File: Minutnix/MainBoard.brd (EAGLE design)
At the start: 222.3 x 73.3 mm, 121 parts, among them IC3 TP4056, IC7 FT232RL, Q4 32.768kHz, X1 FH12-12S-0.5S_THINNER, X2 JST-XH-03-PIN-LONG-PAD, X4 JST-XH-03-PIN-LONG-PAD

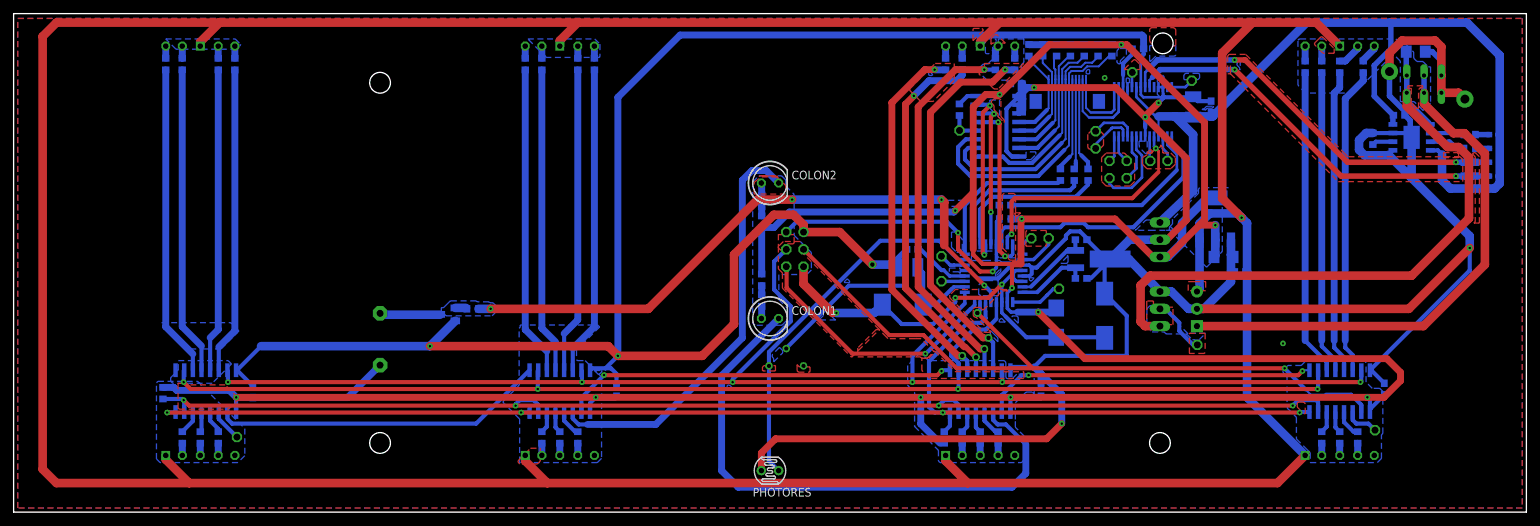
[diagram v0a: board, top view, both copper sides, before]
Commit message: Many final changes
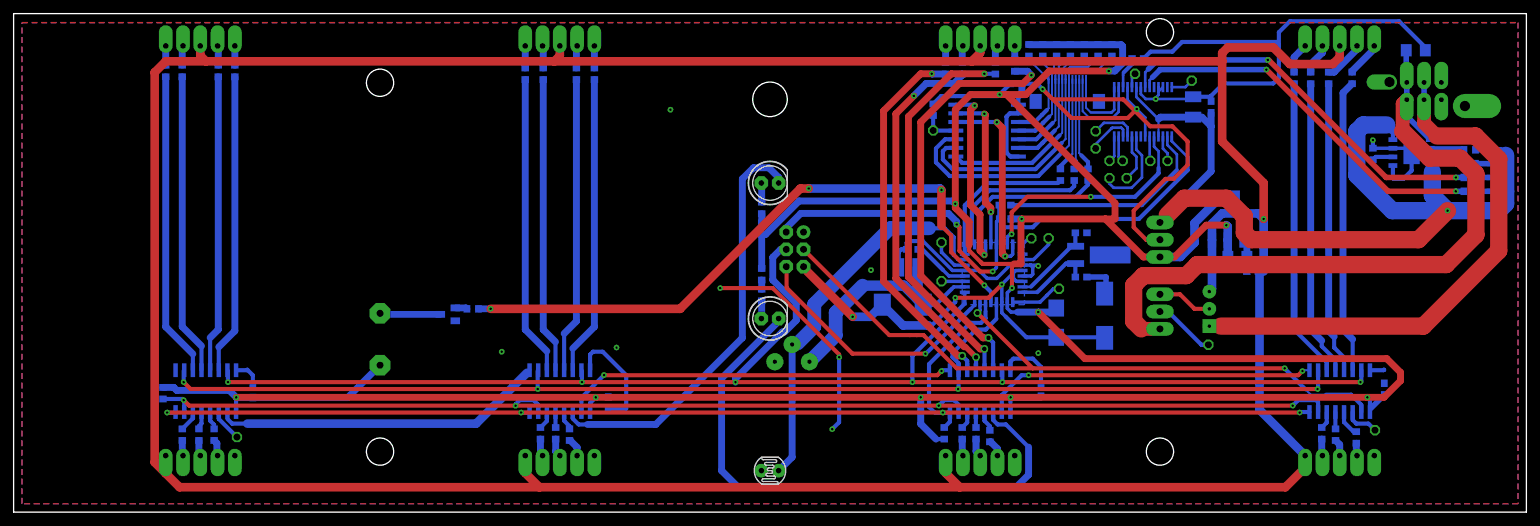
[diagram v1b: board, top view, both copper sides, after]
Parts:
- removed IC2: (no value), v-reg-2:SOT223
- removed IC3: TP4056, TP4056:SOP-8
- removed Q4: 32.768kHz, crystal_clock:CRYSTAL-SMD-2X6-CYL
- removed R57: (no value), rcl:RTRIM3296Y
- removed SG1: F/HGP, buzzer:F/HGP
- removed X2: JST-XH-03-PIN-LONG-PAD, Rembrandt Electronics - JST XH Connectors v1-0:JST-XH-03-PACKAGE-LONG-PAD
- added BATTERY_CON: JST-XH-03-PIN-LONG-PAD, Rembrandt Electronics - JST XH Connectors v1-0:JST-XH-03-PACKAGE-LONG-PAD
- added BUZZER: F/HGP, Mybuzzer:F/HGP
- added CHARGER: TP4056, TP4056:SOP-8
- added LDO_5V: (no value), v-reg-2:SOT223
- added POTENTIOMETER: (no value), Myrcl:RTRIM3296Y
- added QUARTZ: 32.768kHz, crystal_clock:CRYSTAL-SMD-2X6-CYL
- COLON1, COLON2: device led:LED5MM -> Myled:LED5MM
- EXPANDER: value PCF8574AT -> PCF8574T; device i2c:SO16 -> micro-philips:SO16W
- PHOTORES: device photo-elements:VT900 -> Myphoto-elements:VT900
- SPI_JUMPERS: device con-lstb:MA03-2 -> Mycon-lstb:MA03-2
- moved JP6 3.86 mm to (135.1, 56.1)
- moved R61 3.86 mm to (135.1, 59.1)
- moved R15 2.30 mm to (188.2, 63.8)
- moved R16 2.30 mm to (190.6, 63.8)
- moved R20 2.30 mm to (196.7, 63.8)
- moved R21 2.30 mm to (193.2, 63.8)
- moved C2 2.24 mm to (203.6, 56.1)
- moved CHRG_LED 2.24 mm to (217.6, 51.2)
- moved R39 2.24 mm to (214.0, 51.2)
- moved R40 2.24 mm to (214.0, 53.2)
- moved R48 2.24 mm to (199.7, 52.6)
- moved R65 2.24 mm to (214.0, 49.2)
- moved R66 2.24 mm to (214.0, 47.1)
- moved RXLED 2.24 mm to (217.6, 49.2)
- moved STDBY_LED 2.24 mm to (217.6, 53.2)
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- renumbered IC7 to FTDI, Q2 to NPN_AMP, SHOTTKYDIODE3 to SHOTTKY, X1 to FFC_CON, X4 to POWER_CON
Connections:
- net +5V: now also CHARGER.4, CHARGER.8; no longer IC3.4, IC3.8
- net AVCC: now also POTENTIOMETER.1; no longer R57.2
- net BATTERY+: now also BATTERY_CON.1, CHARGER.5; no longer IC3.5, X2.1
- net BATTERY_S: now also BATTERY_CON.2; no longer X2.2
- net COUNTER: now also EXPANDER.9, FFC_CON.8, R42.2; no longer EXPANDER.6, FFC_CON.10, R44.2
- net GND: now also BATTERY_CON.3, CHARGER.1, CHARGER.3, CHARGER.ETP, LDO_5V.1, QUARTZ.SHEILD; no longer FFC_CON.CASE1, FFC_CON.CASE2, IC2.1, IC3.1, IC3.3, IC3.ETP, Q4.SHEILD, X2.3
- net LIGHT_SENS: now also POTENTIOMETER.2; no longer R57.3
- net N$52: now also CHARGER.7; no longer IC3.7
- net N$53: now also CHARGER.6; no longer IC3.6
- net N$66: now also BUZZER.2; no longer SG1.2
- net N$82: now also CHARGER.2; no longer IC3.2
- net PLAY/PAUSE: now also EXPANDER.4, FFC_CON.12, R46.2; no longer EXPANDER.5, FFC_CON.11, R45.2
- net STOP/RESET: now also EXPANDER.5, FFC_CON.11, R45.2; no longer EXPANDER.4, FFC_CON.12, R46.2
- net VCC: now also BUZZER.1, LDO_5V.2, LDO_5V.4; no longer IC2.2, IC2.4, SG1.1
- net VDD: now also LDO_5V.3; no longer IC2.3
- net VOLUME: now also EXPANDER.6, FFC_CON.10, R44.2; no longer EXPANDER.9, FFC_CON.8, R42.2
- net XTAL1: now also QUARTZ.X2; no longer Q4.X2
- net XTAL2: now also QUARTZ.X1; no longer Q4.X1
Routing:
- net GND: track 668.0 -> 296.4 mm, vias 10 -> 13
- net VDD: track 562.5 -> 514.6 mm
- net COUNTER: track 16.4 -> 31.2 mm
- net VOLUME: track 28.1 -> 16.5 mm
- net BATTERY+: track 96.1 -> 104.8 mm
- net MS_B: track 57.2 -> 63.1 mm
- net N$27: track 8.33 -> 4.74 mm
- net ENC_A: track 36.2 -> 39.5 mm
- net ENC_B: track 42.6 -> 45.7 mm
- net EXP_INT: track 25.9 -> 28.9 mm
- net LIGHT_SENS: track 54.7 -> 57.2 mm
- net N$42: track 2.20 -> 4.59 mm
- net N$48: track 3.77 -> 6.11 mm
- net N$47: track 2.87 -> 5.20 mm
- net N$41: track 2.20 -> 4.52 mm
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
